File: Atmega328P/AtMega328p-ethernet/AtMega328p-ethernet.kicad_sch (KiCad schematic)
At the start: 18 parts, among them J1 Conn_01x05_Socket, J4 Conn_01x06_Socket, J5 Conn_01x06_Socket, J6 Conn_01x04_Socket, SW1 SW_Push, U1 ATmega328P-A, Y1 16MHz

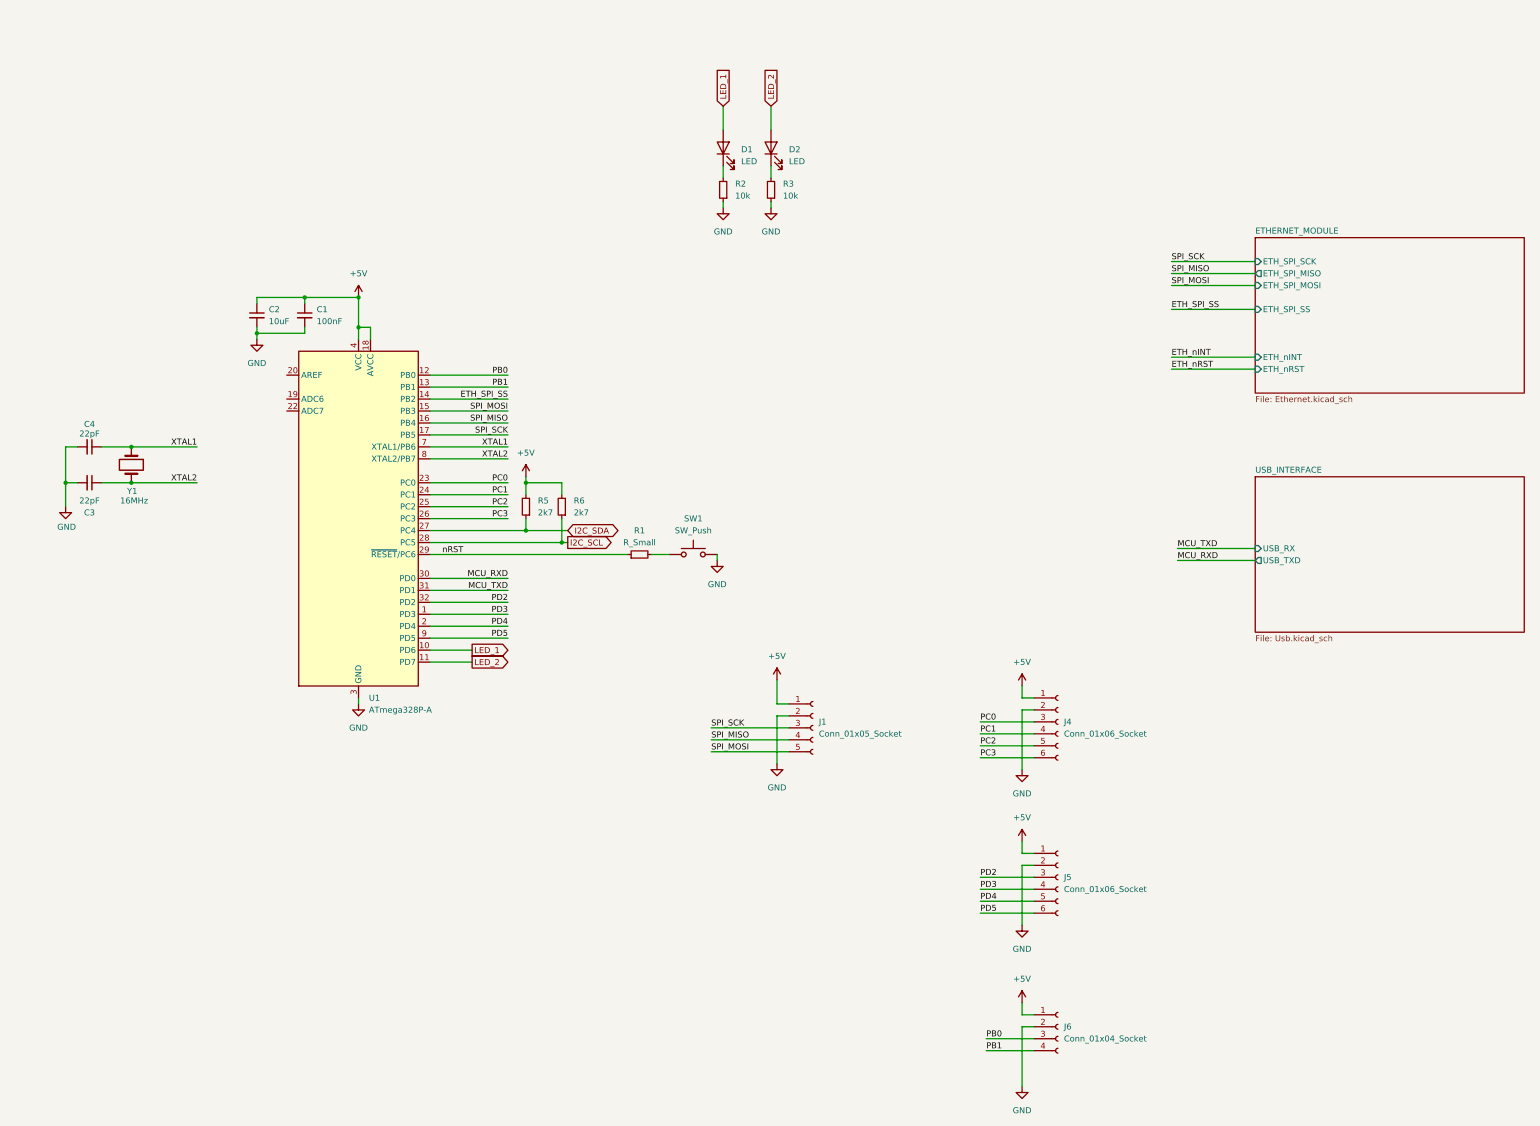
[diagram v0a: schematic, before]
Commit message: Schematic draft complete
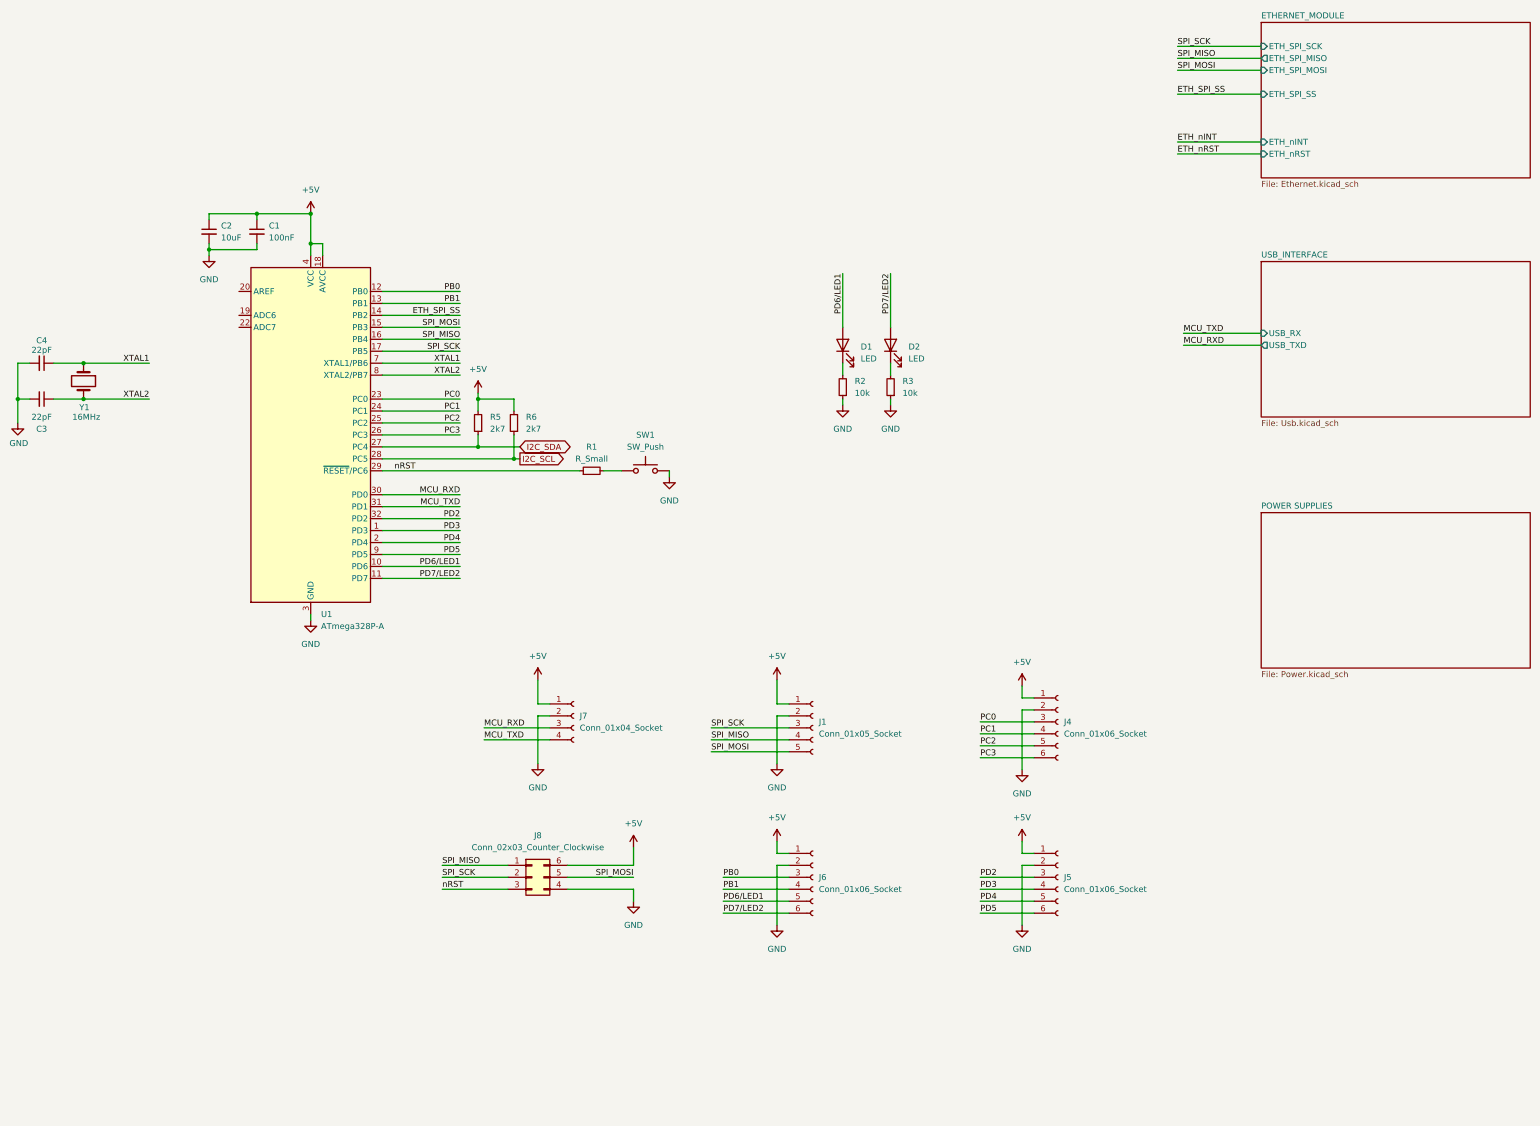
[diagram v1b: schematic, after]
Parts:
- removed J6: Conn_01x04_Socket, symbol Connector:Conn_01x04_Socket
- added J6: Conn_01x06_Socket, Connector_PinHeader_1.27mm:PinHeader_1x06_P1.27mm_Vertical, symbol Connector:Conn_01x06_Socket
- added J7: Conn_01x04_Socket, Connector_PinHeader_1.27mm:PinHeader_1x04_P1.27mm_Vertical, symbol Connector:Conn_01x04_Socket
- added J8: Conn_02x03_Counter_Clockwise, Connector_PinHeader_1.27mm:PinHeader_2x03_P1.27mm_Vertical, symbol Connector_Generic:Conn_02x03_Counter_Clockwise
- C1, C3, C4: footprint (none) -> Capacitor_SMD:C_0603_1608Metric
- C2: footprint (none) -> Capacitor_SMD:CP_Elec_4x3
- D1, D2: footprint (none) -> LED_SMD:LED_0603_1608Metric
- J1: footprint (none) -> Connector_PinHeader_1.27mm:PinHeader_1x05_P1.27mm_Vertical
- J4, J5: footprint (none) -> Connector_PinHeader_1.27mm:PinHeader_1x06_P1.27mm_Vertical
- R1, R2, R3, R5, R6: footprint (none) -> Resistor_SMD:R_0603_1608Metric
- SW1: footprint (none) -> Button_Switch_SMD:SW_Push_1P1T_NO_CK_KMR2
- Y1: footprint (none) -> Crystal:Crystal_SMD_2012-2Pin_2.0x1.2mm
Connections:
- net +5V: now also J6.1 (Pin_1), J7.1 (Pin_1), J8.6 (Pin_6)
- net GND: now also J6.2 (Pin_2), J7.2 (Pin_2), J8.4 (Pin_4)
- net MCU_RXD: now also J7.3 (Pin_3)
- net MCU_TXD: now also J7.4 (Pin_4)
- net PB0: now also J6.3 (Pin_3)
- net PB1: now also J6.4 (Pin_4)
- net SPI_MISO: now also J8.1 (Pin_1)
- net SPI_MOSI: now also J8.5 (Pin_5)
- net SPI_SCK: now also J8.2 (Pin_2)
- net nRST: now also J8.3 (Pin_3)
- net LED_1 renamed PD6/LED1
- net PD6/LED1: now also J6.5 (Pin_5)
- net LED_2 renamed PD7/LED2
- net PD7/LED2: now also J6.6 (Pin_6)
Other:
- added sheet POWER SUPPLIES (Power.kicad_sch)
- company: (none) -> HUNTER INC.
- title: (none) -> MAIN SHEET
- moved on the sheet: C1, C2, C3, C4, D1, D2, R1, R2, R3, R5, R6, SW1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

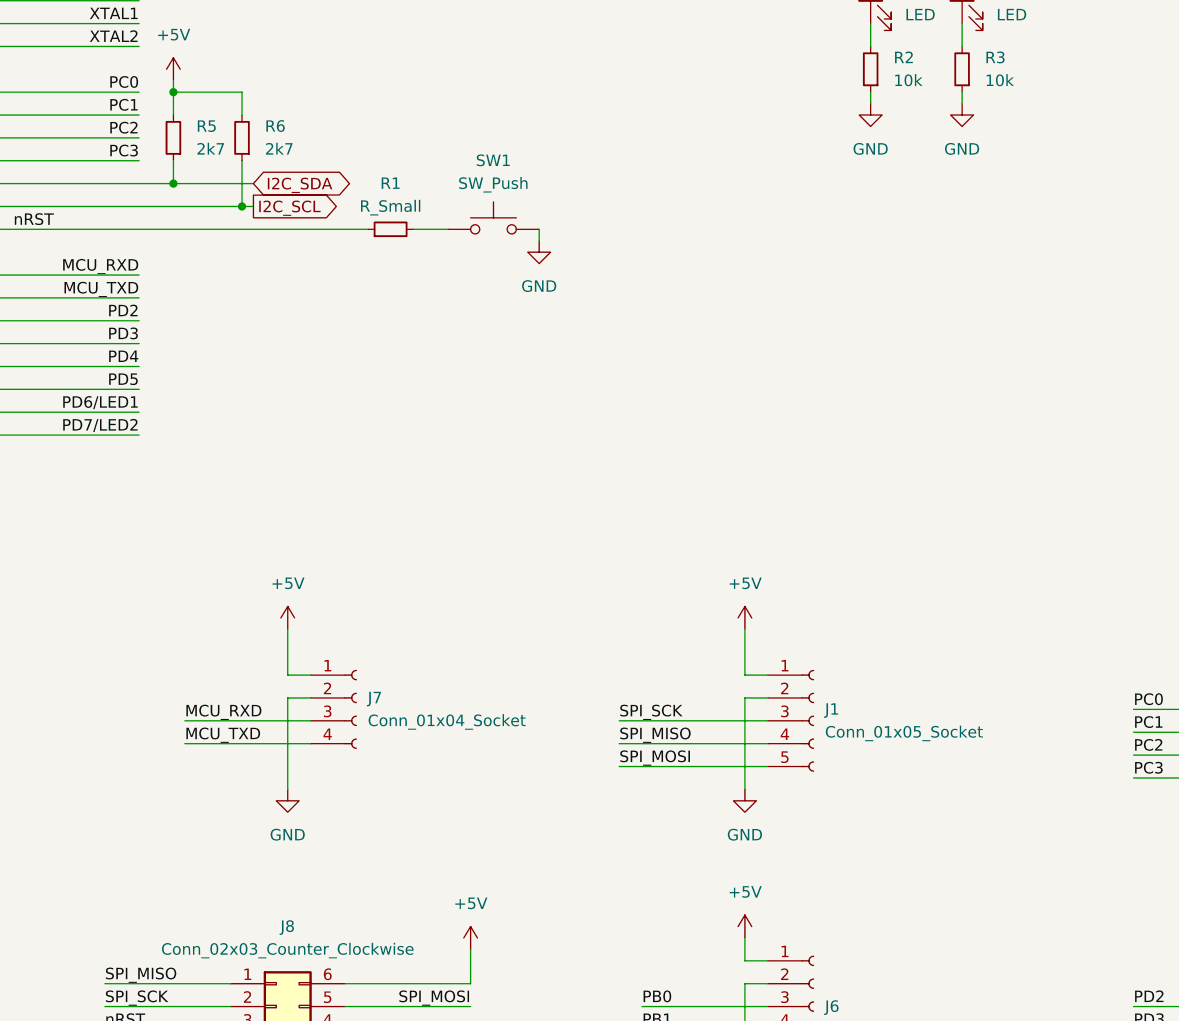
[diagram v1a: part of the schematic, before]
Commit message: PCB Layout done initial
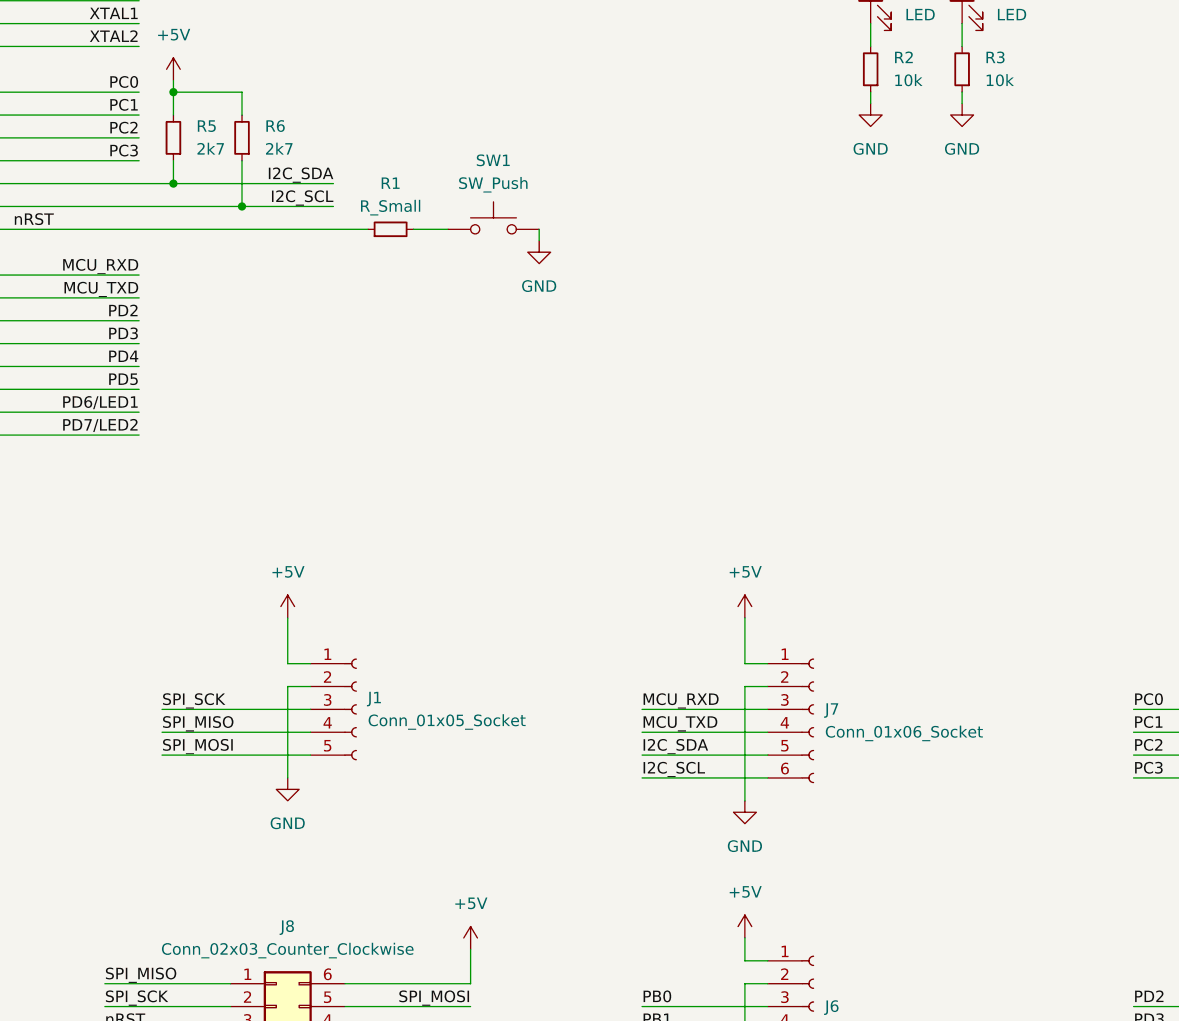
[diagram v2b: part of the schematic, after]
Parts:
- removed J7: Conn_01x04_Socket, Connector_PinHeader_1.27mm:PinHeader_1x04_P1.27mm_Vertical, symbol Connector:Conn_01x04_Socket
- added J7: Conn_01x06_Socket, Connector_PinHeader_2.54mm:PinHeader_1x06_P2.54mm_Vertical, symbol Connector:Conn_01x06_Socket
- J1: footprint Connector_PinHeader_1.27mm:PinHeader_1x05_P1.27mm_Vertical -> Connector_PinHeader_2.54mm:PinHeader_1x05_P2.54mm_Vertical
- J4, J5, J6: footprint Connector_PinHeader_1.27mm:PinHeader_1x06_P1.27mm_Vertical -> Connector_PinHeader_2.54mm:PinHeader_1x06_P2.54mm_Vertical
- J8: footprint Connector_PinHeader_1.27mm:PinHeader_2x03_P1.27mm_Vertical -> Connector_PinHeader_2.54mm:PinHeader_2x03_P2.54mm_Vertical
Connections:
- net +5V: now also J7.1 (Pin_1)
- net GND: now also J7.2 (Pin_2)
- net I2C_SCL: now also J7.6 (Pin_6)
- net I2C_SDA: now also J7.5 (Pin_5)
- net MCU_RXD: now also J7.3 (Pin_3)
- net MCU_TXD: now also J7.4 (Pin_4)
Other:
- moved on the sheet: J1
